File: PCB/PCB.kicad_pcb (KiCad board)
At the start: 4 copper layers, 56.5 x 52.5 mm, 36 parts, among them J1 AudioJack3, J2 AudioJack3, J3 Conn_02x04_Odd_Even, J4 Conn_01x02, J5 Conn_02x04_Odd_Even, Q1 2N7002, Q2 2N7002, Q3 2N7002, Q4 2N7002, U2 LM358

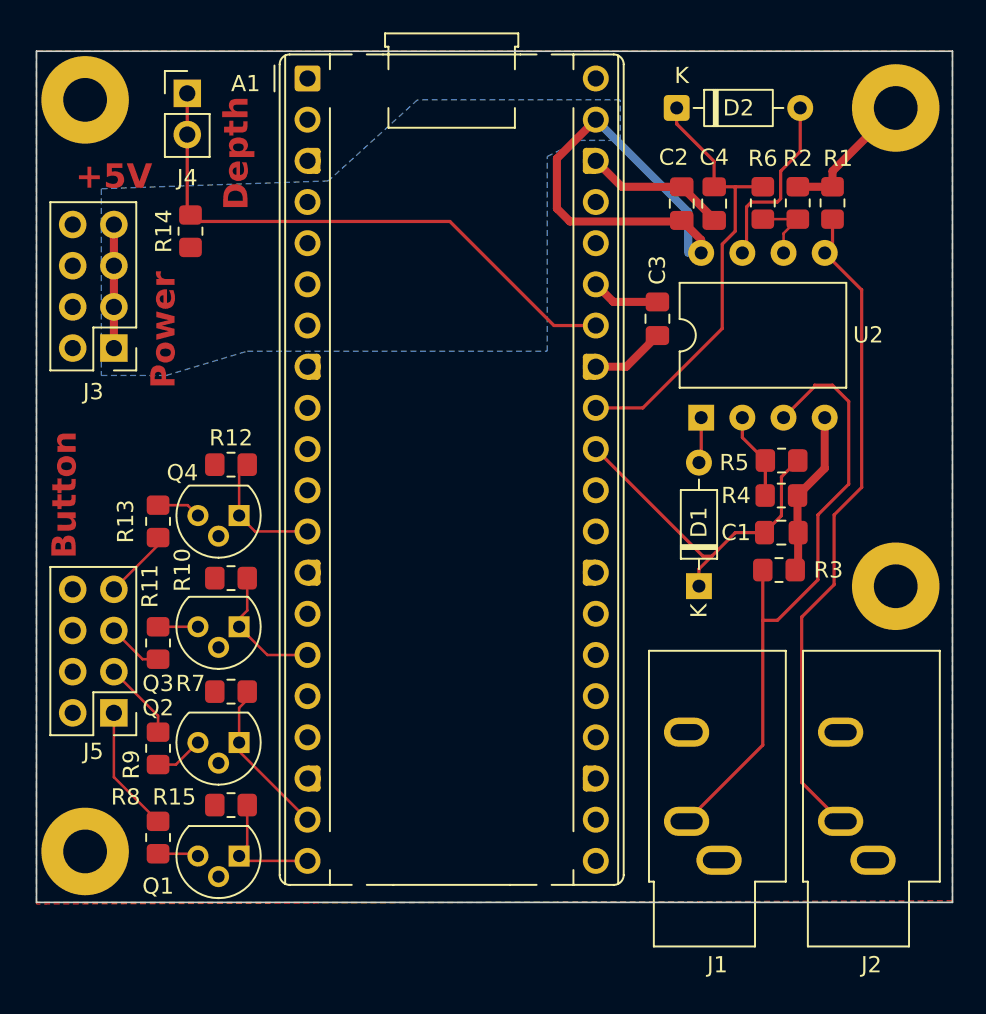
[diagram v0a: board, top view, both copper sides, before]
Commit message: First Spin of PCB
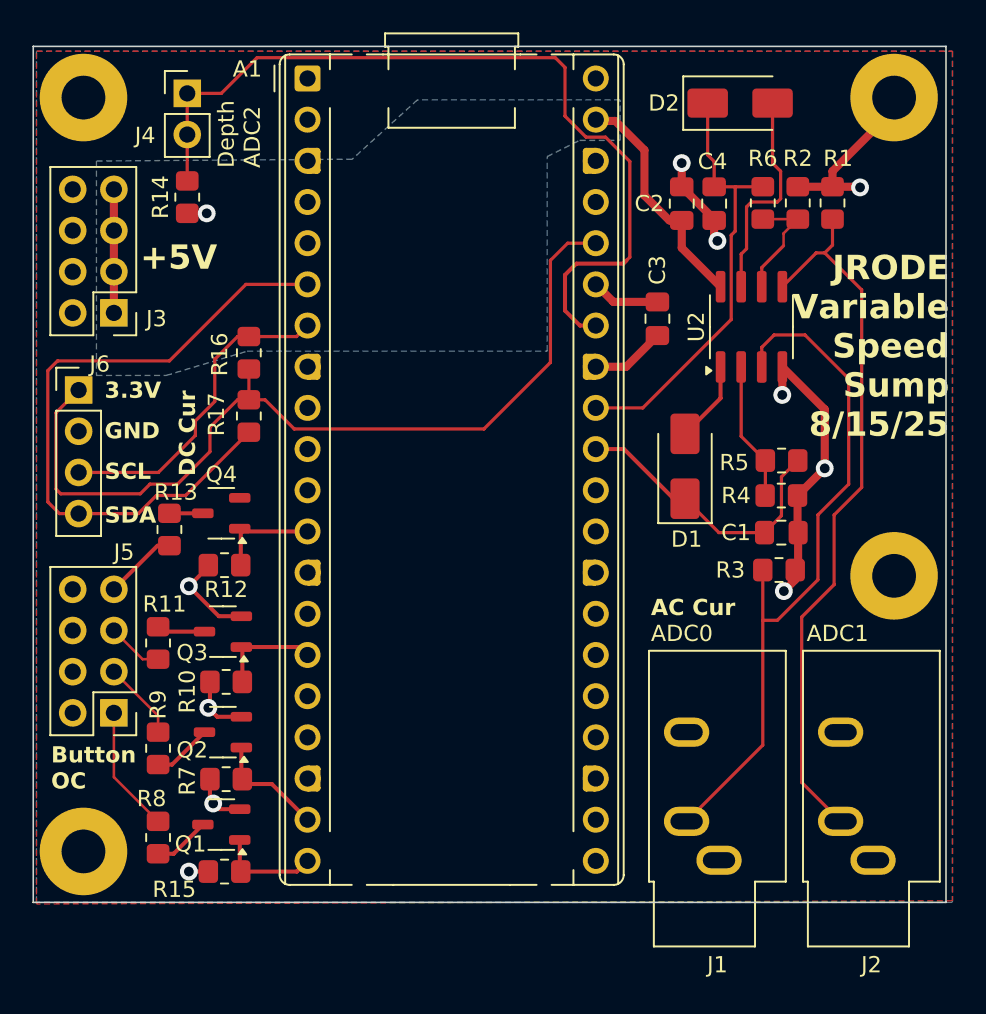
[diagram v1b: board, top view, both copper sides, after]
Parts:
- added J6: Conn_01x04, Connector_PinHeader_2.54mm:PinHeader_1x04_P2.54mm_Vertical, F.Cu at (114.7, 88.5)
- added R16: ~, Resistor_SMD:R_0805_2012Metric_Pad1.20x1.40mm_HandSolder, F.Cu at (125.2, 86.2)
- added R17: ~, Resistor_SMD:R_0805_2012Metric_Pad1.20x1.40mm_HandSolder, F.Cu at (125.2, 90.1)
- C1, C4: value 1u -> 10u
- D1, D2: value BAS33 -> M7; footprint Diode_THT:D_DO-35_SOD27_P7.62mm_Horizontal -> Diode_SMD:D_SMA
- Q1, Q2, Q3, Q4: footprint Package_TO_SOT_THT:TO-92 -> Package_TO_SOT_SMD:SOT-23-3
- R1, R3: value 30 -> 33
- R14: value 165 -> 150
- R2, R4: value 10k -> 470k
- R5, R6: value 22k -> 1M
- U2: footprint Package_DIP:DIP-8_W10.16mm -> Package_SO:SOIC-8_3.9x4.9mm_P1.27mm
- moved D1 7.44 mm to (152.1, 93.2)
- moved R10 6.41 mm to (123.8, 106.5)
- moved U2 6.40 mm to (156.2, 84.6)
- moved R12 6.21 mm to (123.7, 99.3)
- moved R7 5.41 mm to (123.8, 112.5)
- moved R15 4.12 mm to (123.7, 118.2)
- moved D2 3.92 mm to (155.5, 70.8)
- moved Q1 2.23 mm to (123.5, 115.3)
- moved J3 2.17 mm to (116.9, 83.8)
- moved R14 2.11 mm to (121.4, 76.6)
- moved Q2 1.19 mm to (123.6, 109.6)
- moved Q4 1.11 mm to (123.5, 96.1)
- moved Q3 1.04 mm to (123.6, 103.4)
- moved R13 0.86 mm to (120.3, 97.1)
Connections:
- A1 pad 36: unconnected-(A1-3V3-Pad36) -> +3.3V
- A1 pad 4: +5V -> unconnected-(A1-GPIO2-Pad4)
- A1 pad 5: +5V -> unconnected-(A1-GPIO3-Pad5)
- A1 pad 6: +5V -> /SDA
- A1 pad 7: +5V -> /SCL
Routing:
- net +3.3V: track 0.00 -> 54.5 mm
- net /SDA: track 0.00 -> 41.1 mm
- net GND: track 32.3 -> 53.8 mm, vias 0 -> 11
- net /SCL: track 0.00 -> 19.9 mm
- net Net-(A1-GPIO28_ADC2): track 35.4 -> 52.9 mm
- net +5V: track 35.9 -> 22.2 mm
- net Net-(U2A-+): track 39.0 -> 43.1 mm
- net /CT_Input/Output: track 21.2 -> 17.8 mm
- net Net-(U2A--): track 5.40 -> 8.56 mm
- net Net-(U2B-+): track 41.3 -> 44.3 mm
- net /Pull Down1/in: track 9.86 -> 7.03 mm
- net Net-(U2B--): track 4.61 -> 7.25 mm
- net Net-(D1-A): track 2.83 -> 5.03 mm
- net Net-(D2-A): track 11.4 -> 13.5 mm
- net /Pull Down2/in: track 8.15 -> 6.46 mm
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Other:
- board size 56.5 x 52.5 mm -> 56.3 x 52.8 mm
- board text added: "3.3V"
- board text added: "AC Cur"
- board text added: "ADC0"
- board text added: "ADC1"
- board text added: "Button OC"
- board text added: "DC Cur"
- board text added: "Depth ADC2"
- board text added: "Flip Me Over!"
- board text added: "GND"
- board text added: "JRODE Variable Speed Sump 8/15/25"
- board text added: "SCL"
- board text added: "SDA"
- board text removed: "Button"
- board text removed: "Depth"
- board text removed: "Power"
